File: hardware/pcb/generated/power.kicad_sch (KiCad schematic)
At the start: 9 parts, among them J3 PJ-102A, SW13 RA11131100

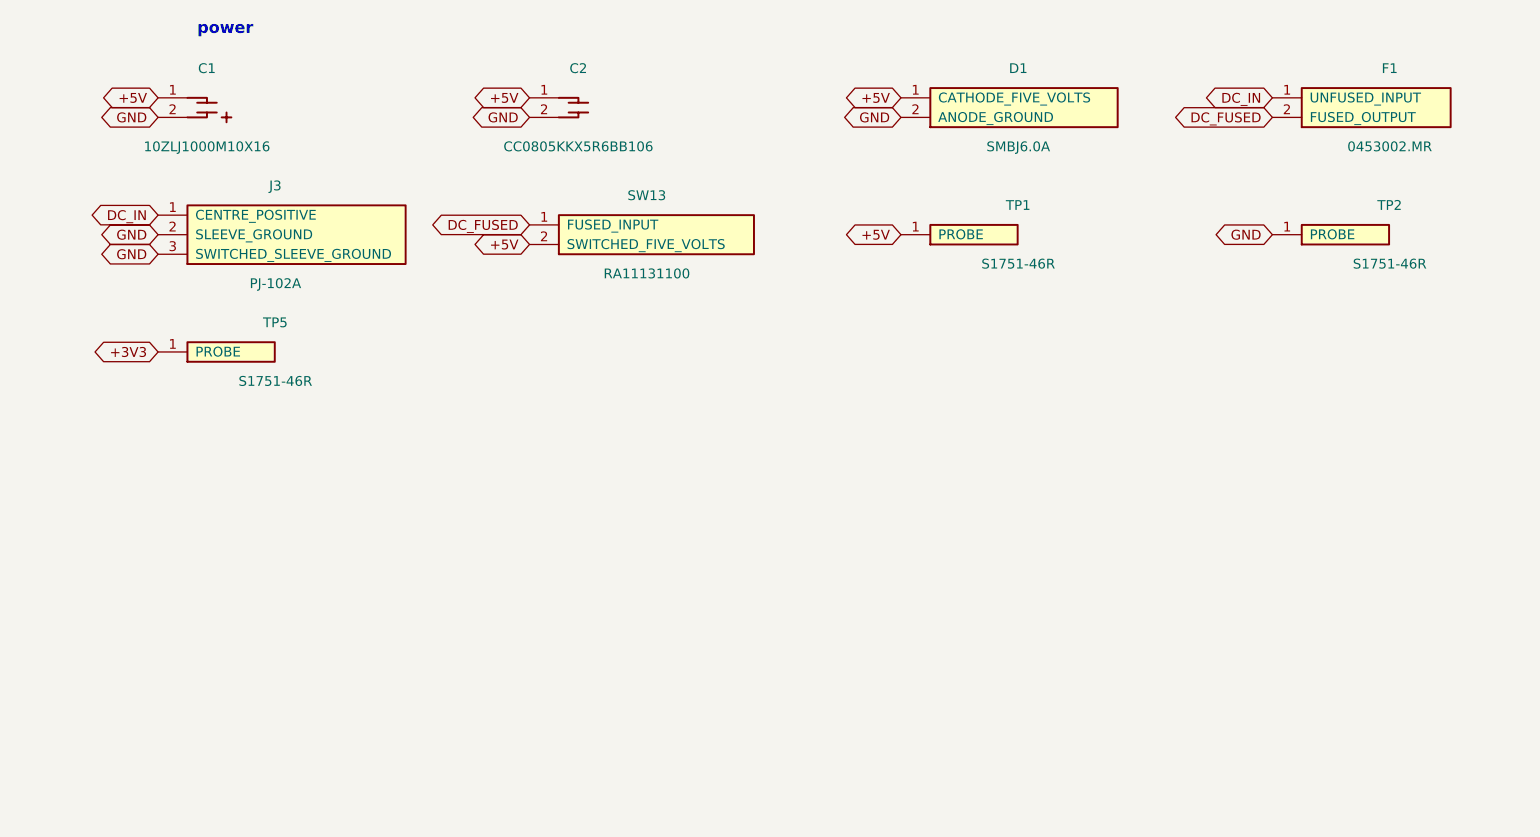
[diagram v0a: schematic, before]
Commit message: chore(pcb): regenerate KiCad, SPICE and review output
Generated by `just pcb` from the committed definition; not hand-edited.
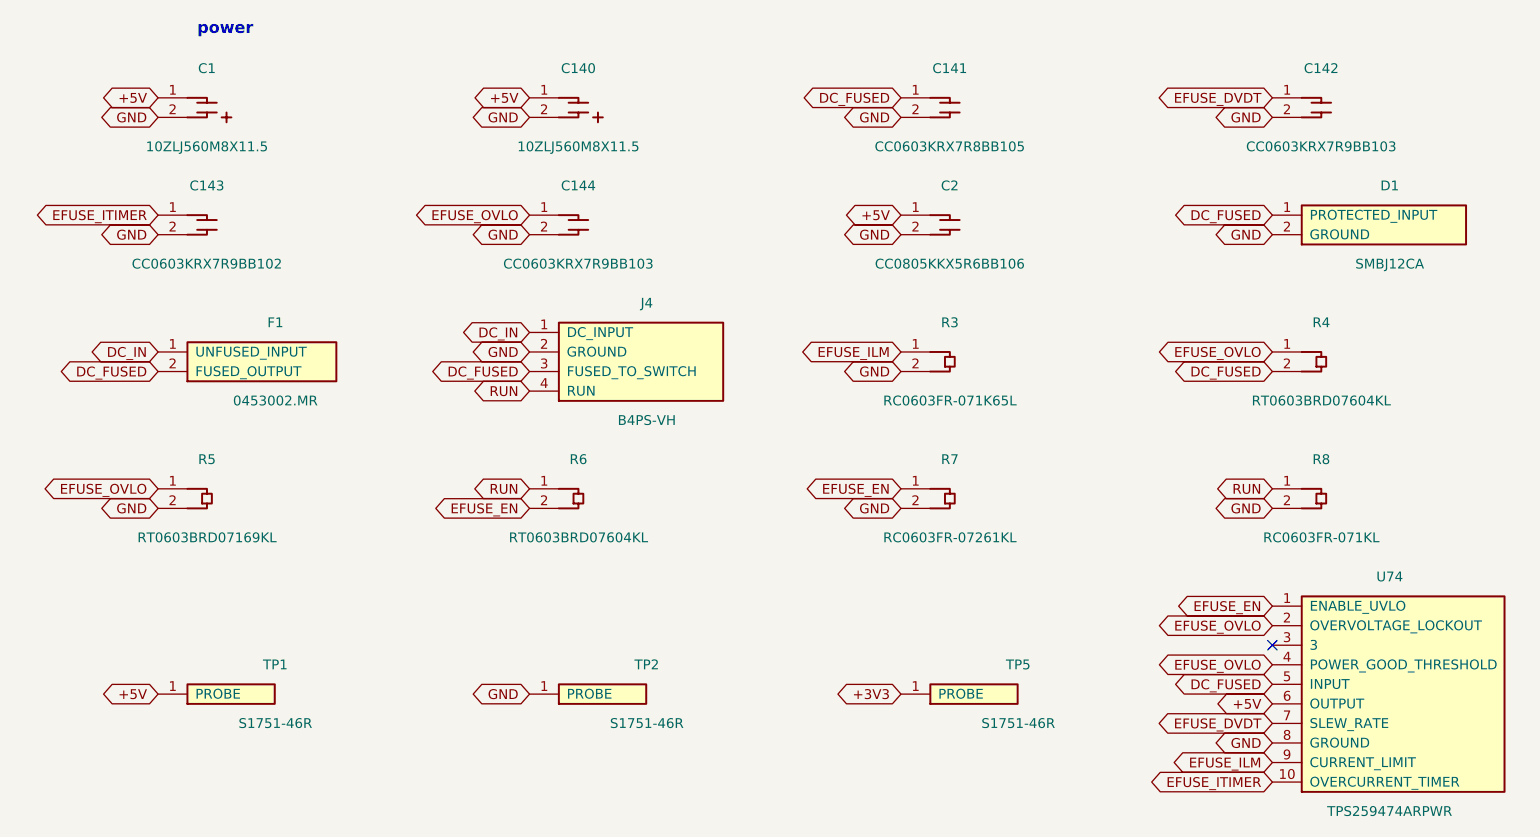
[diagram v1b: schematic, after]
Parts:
- removed J3: PJ-102A, symbol Generated:J3
- removed SW13: RA11131100, symbol Generated:SW13
- added C140: 10ZLJ560M8X11.5, symbol Generated:C140
- added C141: CC0603KRX7R8BB105, symbol Generated:C141
- added C142: CC0603KRX7R9BB103, symbol Generated:C142
- added C143: CC0603KRX7R9BB102, symbol Generated:C143
- added C144: CC0603KRX7R9BB103, symbol Generated:C144
- added J4: B4PS-VH, symbol Generated:J4
- added R3: RC0603FR-071K65L, symbol Generated:R3
- added R4: RT0603BRD07604KL, symbol Generated:R4
- added R5: RT0603BRD07169KL, symbol Generated:R5
- added R6: RT0603BRD07604KL, symbol Generated:R6
- added R7: RC0603FR-07261KL, symbol Generated:R7
- added R8: RC0603FR-071KL, symbol Generated:R8
- added U74: TPS259474ARPWR, symbol Generated:U74
- C1: value 10ZLJ1000M10X16 -> 10ZLJ560M8X11.5
- D1: value SMBJ6.0A -> SMBJ12CA
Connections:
- net +5V: now also C140.1 (SUPPLY_OR_ELECTRODE_A), U74.6 (OUTPUT); no longer D1.1 (CATHODE_FIVE_VOLTS)
- net DC_FUSED: now also D1.1 (PROTECTED_INPUT), C141.1 (SUPPLY_OR_ELECTRODE_A), J4.3 (FUSED_TO_SWITCH), R4.2 (TERMINAL_B), U74.5 (INPUT)
- net DC_IN: now also J4.1 (DC_INPUT)
- net GND: now also C140.2 (RETURN_OR_ELECTRODE_B), C141.2 (RETURN_OR_ELECTRODE_B), C142.2 (RETURN_OR_ELECTRODE_B), C143.2 (RETURN_OR_ELECTRODE_B), C144.2 (RETURN_OR_ELECTRODE_B), J4.2 (GROUND), R3.2 (TERMINAL_B), R5.2 (TERMINAL_B), R7.2 (TERMINAL_B), R8.2 (TERMINAL_B), U74.8 (GROUND)
- new net EFUSE_DVDT: C142.1 (SUPPLY_OR_ELECTRODE_A), U74.7 (SLEW_RATE)
- new net EFUSE_EN: R6.2 (TERMINAL_B), R7.1 (TERMINAL_A), U74.1 (ENABLE_UVLO)
- new net EFUSE_ILM: R3.1 (TERMINAL_A), U74.9 (CURRENT_LIMIT)
- new net EFUSE_ITIMER: C143.1 (SUPPLY_OR_ELECTRODE_A), U74.10 (OVERCURRENT_TIMER)
- new net EFUSE_OVLO: C144.1 (SUPPLY_OR_ELECTRODE_A), R4.1 (TERMINAL_A), R5.1 (TERMINAL_A), U74.2 (OVERVOLTAGE_LOCKOUT), U74.4 (POWER_GOOD_THRESHOLD)
- new net RUN: J4.4 (RUN), R6.1 (TERMINAL_A), R8.1 (TERMINAL_A)
- no-connect marks 0 -> 1
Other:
- moved on the sheet: C2, D1, F1, TP1, TP2, TP5
